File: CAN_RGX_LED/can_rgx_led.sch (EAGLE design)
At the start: 9 parts

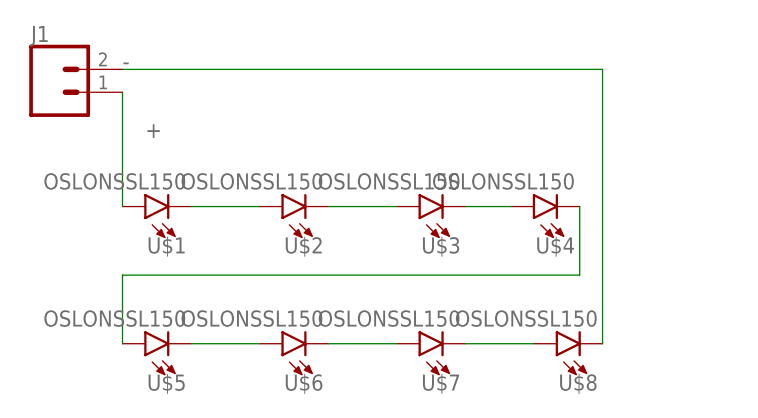
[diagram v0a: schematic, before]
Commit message: board 1_0
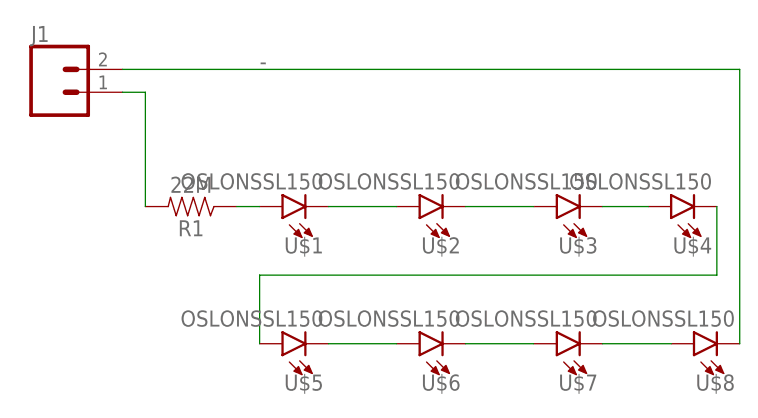
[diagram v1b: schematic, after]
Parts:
- added R1: 22M, SparkFun-Resistors:22MOHM-0603-1/10W-10%
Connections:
- new net N$8: R1.1, U$1.A
- net +: now also R1.2; no longer U$1.A
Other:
- moved on the sheet: U$1, U$2, U$3, U$4, U$5, U$6, U$7, U$8
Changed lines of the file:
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@@
 <part name="U$8" library="uORocketry-parts" deviceset="OSLONSSL150" device=""/>
 <part name="J1" library="SparkFun-Connectors" deviceset="CONN_02" device=""/>
+<part name="R1" library="SparkFun-Resistors" deviceset="22MOHM" device="-0603-1/10W-10%" value="22M"/>
 </parts>
 <sheets>
@@
 </plain>
 <instances>
-<instance part="U$1" gate="G$1" x="33.02" y="55.88" smashed="yes">
-<attribute name="NAME" x="32.512" y="52.451" size="1.778" layer="95" font="vector" rot="R180"/>
-<attribute name="VALUE" x="32.512" y="57.785" size="1.778" layer="96" font="vector" rot="R180" align="top-left"/>
-</instance>
-<instance part="U$2" gate="G$1" x="48.26" y="55.88" smashed="yes">
+<instance part="U$1" gate="G$1" x="48.26" y="55.88" smashed="yes">
 <attribute name="NAME" x="47.752" y="52.451" size="1.778" layer="95" font="vector" rot="R180"/>
 <attribute name="VALUE" x="47.752" y="57.785" size="1.778" layer="96" font="vector" rot="R180" align="top-left"/>
 </instance>
-<instance part="U$3" gate="G$1" x="63.5" y="55.88" smashed="yes">
+<instance part="U$2" gate="G$1" x="63.5" y="55.88" smashed="yes">
 <attribute name="NAME" x="62.992" y="52.451" size="1.778" layer="95" font="vector" rot="R180"/>
 <attribute name="VALUE" x="62.992" y="57.785" size="1.778" layer="96" font="vector" rot="R180" align="top-left"/>
 </instance>
-<instance part="U$4" gate="G$1" x="76.2" y="55.88" smashed="yes">
-<attribute name="NAME" x="75.692" y="52.451" size="1.778" layer="95" font="vector" rot="R180"/>
-<attribute name="VALUE" x="75.692" y="57.785" size="1.778" layer="96" font="vector" rot="R180" align="top-left"/>
+<instance part="U$3" gate="G$1" x="78.74" y="55.88" smashed="yes">
+<attribute name="NAME" x="78.232" y="52.451" size="1.778" layer="95" font="vector" rot="R180"/>
+<attribute name="VALUE" x="78.232" y="57.785" size="1.778" layer="96" font="vector" rot="R180" align="top-left"/>
 </instance>
-<instance part="U$5" gate="G$1" x="33.02" y="40.64" smashed="yes">
-<attribute name="NAME" x="32.512" y="37.211" size="1.778" layer="95" font="vector" rot="R180"/>
-<attribute name="VALUE" x="32.512" y="42.545" size="1.778" layer="96" font="vector" rot="R180" align="top-left"/>
+<instance part="U$4" gate="G$1" x="91.44" y="55.88" smashed="yes">
+<attribute name="NAME" x="90.932" y="52.451" size="1.778" layer="95" font="vector" rot="R180"/>
+<attribute name="VALUE" x="90.932" y="57.785" size="1.778" layer="96" font="vector" rot="R180" align="top-left"/>
 </instance>
-<instance part="U$6" gate="G$1" x="48.26" y="40.64" smashed="yes">
+<instance part="U$5" gate="G$1" x="48.26" y="40.64" smashed="yes">
 <attribute name="NAME" x="47.752" y="37.211" size="1.778" layer="95" font="vector" rot="R180"/>
 <attribute name="VALUE" x="47.752" y="42.545" size="1.778" layer="96" font="vector" rot="R180" align="top-left"/>
 </instance>
-<instance part="U$7" gate="G$1" x="63.5" y="40.64" smashed="yes">
+<instance part="U$6" gate="G$1" x="63.5" y="40.64" smashed="yes">
 <attribute name="NAME" x="62.992" y="37.211" size="1.778" layer="95" font="vector" rot="R180"/>
 <attribute name="VALUE" x="62.992" y="42.545" size="1.778" layer="96" font="vector" rot="R180" align="top-left"/>
 </instance>
-<instance part="U$8" gate="G$1" x="78.74" y="40.64" smashed="yes">
+<instance part="U$7" gate="G$1" x="78.74" y="40.64" smashed="yes">
 <attribute name="NAME" x="78.232" y="37.211" size="1.778" layer="95" font="vector" rot="R180"/>
 <attribute name="VALUE" x="78.232" y="42.545" size="1.778" layer="96" font="vector" rot="R180" align="top-left"/>
+</instance>
+<instance part="U$8" gate="G$1" x="93.98" y="40.64" smashed="yes">
+<attribute name="NAME" x="93.472" y="37.211" size="1.778" layer="95" font="vector" rot="R180"/>
+<attribute name="VALUE" x="93.472" y="42.545" size="1.778" layer="96" font="vector" rot="R180" align="top-left"/>
 </instance>
 <instance part="J1" gate="G$1" x="17.78" y="68.58" smashed="yes">
 <attribute name="VALUE" x="15.24" y="63.754" size="1.778" layer="96" font="vector"/>
 <attribute name="NAME" x="15.24" y="74.168" size="1.778" layer="95" font="vector"/>
+</instance>
+<instance part="R1" gate="G$1" x="33.02" y="55.88" smashed="yes" rot="R180">
+<attribute name="NAME" x="33.02" y="54.356" size="1.778" layer="95" font="vector" rot="R180" align="bottom-center"/>
+<attribute name="VALUE" x="33.02" y="57.404" size="1.778" layer="96" font="vector" rot="R180" align="top-center"/>
 </instance>
 </instances>
@@
 <pinref part="U$1" gate="G$1" pin="C"/>
 <pinref part="U$2" gate="G$1" pin="A"/>
-<wire x1="33.02" y1="55.88" x2="40.64" y2="55.88" width="0.1524" layer="91"/>
+<wire x1="48.26" y1="55.88" x2="55.88" y2="55.88" width="0.1524" layer="91"/>
 </segment>
 </net>
@@
 <pinref part="U$2" gate="G$1" pin="C"/>
 <pinref part="U$3" gate="G$1" pin="A"/>
-<wire x1="48.26" y1="55.88" x2="55.88" y2="55.88" width="0.1524" layer="91"/>
+<wire x1="63.5" y1="55.88" x2="71.12" y2="55.88" width="0.1524" layer="91"/>
 </segment>
 </net>
@@
 <pinref part="U$3" gate="G$1" pin="C"/>
 <pinref part="U$4" gate="G$1" pin="A"/>
-<wire x1="63.5" y1="55.88" x2="68.58" y2="55.88" width="0.1524" layer="91"/>
+<wire x1="78.74" y1="55.88" x2="83.82" y2="55.88" width="0.1524" layer="91"/>
 </segment>
 </net>
@@
 <segment>
 <pinref part="U$4" gate="G$1" pin="C"/>
-<wire x1="76.2" y1="55.88" x2="76.2" y2="48.26" width="0.1524" layer="91"/>
-<wire x1="76.2" y1="48.26" x2="25.4" y2="48.26" width="0.1524" layer="91"/>
+<wire x1="91.44" y1="55.88" x2="91.44" y2="48.26" width="0.1524" layer="91"/>
+<wire x1="91.44" y1="48.26" x2="40.64" y2="48.26" width="0.1524" layer="91"/>
 <pinref part="U$5" gate="G$1" pin="A"/>
-<wire x1="25.4" y1="48.26" x2="25.4" y2="40.64" width="0.1524" layer="91"/>
+<wire x1="40.64" y1="48.26" x2="40.64" y2="40.64" width="0.1524" layer="91"/>
 </segment>
 </net>
@@
 <pinref part="U$5" gate="G$1" pin="C"/>
 <pinref part="U$6" gate="G$1" pin="A"/>
-<wire x1="33.02" y1="40.64" x2="40.64" y2="40.64" width="0.1524" layer="91"/>
+<wire x1="48.26" y1="40.64" x2="55.88" y2="40.64" width="0.1524" layer="91"/>
 </segment>
 </net>
@@
 <pinref part="U$6" gate="G$1" pin="C"/>
 <pinref part="U$7" gate="G$1" pin="A"/>
-<wire x1="48.26" y1="40.64" x2="55.88" y2="40.64" width="0.1524" layer="91"/>
+<wire x1="63.5" y1="40.64" x2="71.12" y2="40.64" width="0.1524" layer="91"/>
 </segment>
 </net>
@@
 <pinref part="U$7" gate="G$1" pin="C"/>
 <pinref part="U$8" gate="G$1" pin="A"/>
-<wire x1="63.5" y1="40.64" x2="71.12" y2="40.64" width="0.1524" layer="91"/>
-</segment>
-</net>
-<net name="+" class="0">
-<segment>
-<pinref part="J1" gate="G$1" pin="1"/>
-<pinref part="U$1" gate="G$1" pin="A"/>
-<wire x1="25.4" y1="68.58" x2="25.4" y2="55.88" width="0.1524" layer="91"/>
-<label x="27.94" y="63.5" size="1.778" layer="95"/>
+<wire x1="78.74" y1="40.64" x2="86.36" y2="40.64" width="0.1524" layer="91"/>
 </segment>
 </net>
@@
 <pinref part="J1" gate="G$1" pin="2"/>
 <pinref part="U$8" gate="G$1" pin="C"/>
-<wire x1="25.4" y1="71.12" x2="78.74" y2="71.12" width="0.1524" layer="91"/>
-<wire x1="78.74" y1="71.12" x2="78.74" y2="40.64" width="0.1524" layer="91"/>
-<label x="25.4" y="71.12" size="1.778" layer="95"/>
+<wire x1="25.4" y1="71.12" x2="93.98" y2="71.12" width="0.1524" layer="91"/>
+<wire x1="93.98" y1="71.12" x2="93.98" y2="40.64" width="0.1524" layer="91"/>
+<label x="40.64" y="71.12" size="1.778" layer="95"/>
 </segment>
 </net>
+<net name="N$8" class="0">
+<segment>
+<pinref part="R1" gate="G$1" pin="1"/>
+<pinref part="U$1" gate="G$1" pin="A"/>
+<wire x1="38.1" y1="55.88" x2="40.64" y2="55.88" width="0.1524" layer="91"/>
+</segment>
+</net>
+<net name="+" class="0">
+<segment>
+<pinref part="R1" gate="G$1" pin="2"/>
+<pinref part="J1" gate="G$1" pin="1"/>
+<wire x1="27.94" y1="55.88" x2="27.94" y2="68.58" width="0.1524" layer="91"/>
+<wire x1="27.94" y1="68.58" x2="25.4" y2="68.58" width="0.1524" layer="91"/>
+</segment>
+</net>
